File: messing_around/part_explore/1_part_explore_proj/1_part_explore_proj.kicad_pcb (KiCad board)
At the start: 2 copper layers, 8.2 x 5 mm, 2 parts, among them P1 USB_C_Plug_USB2.0, U1 ESP32-C3-WROOM-02

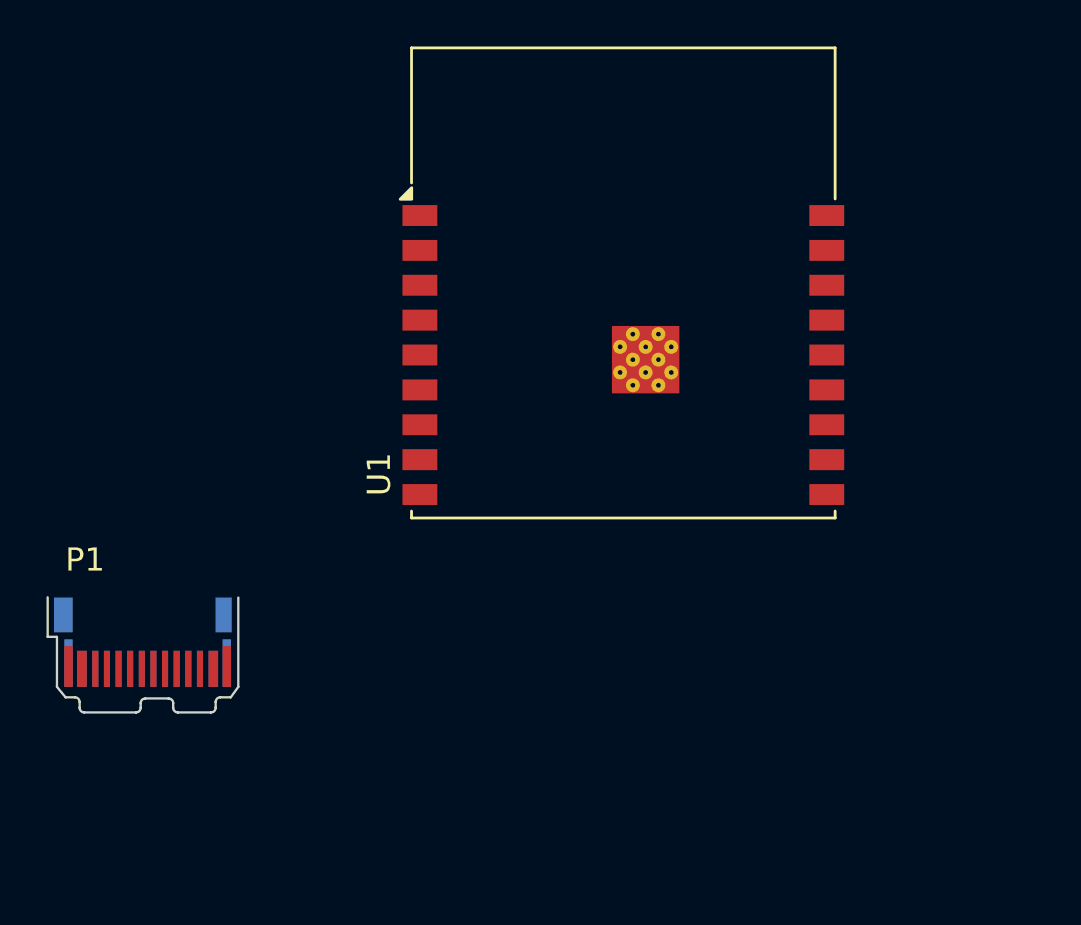
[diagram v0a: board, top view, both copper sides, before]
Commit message: messing around with the settings
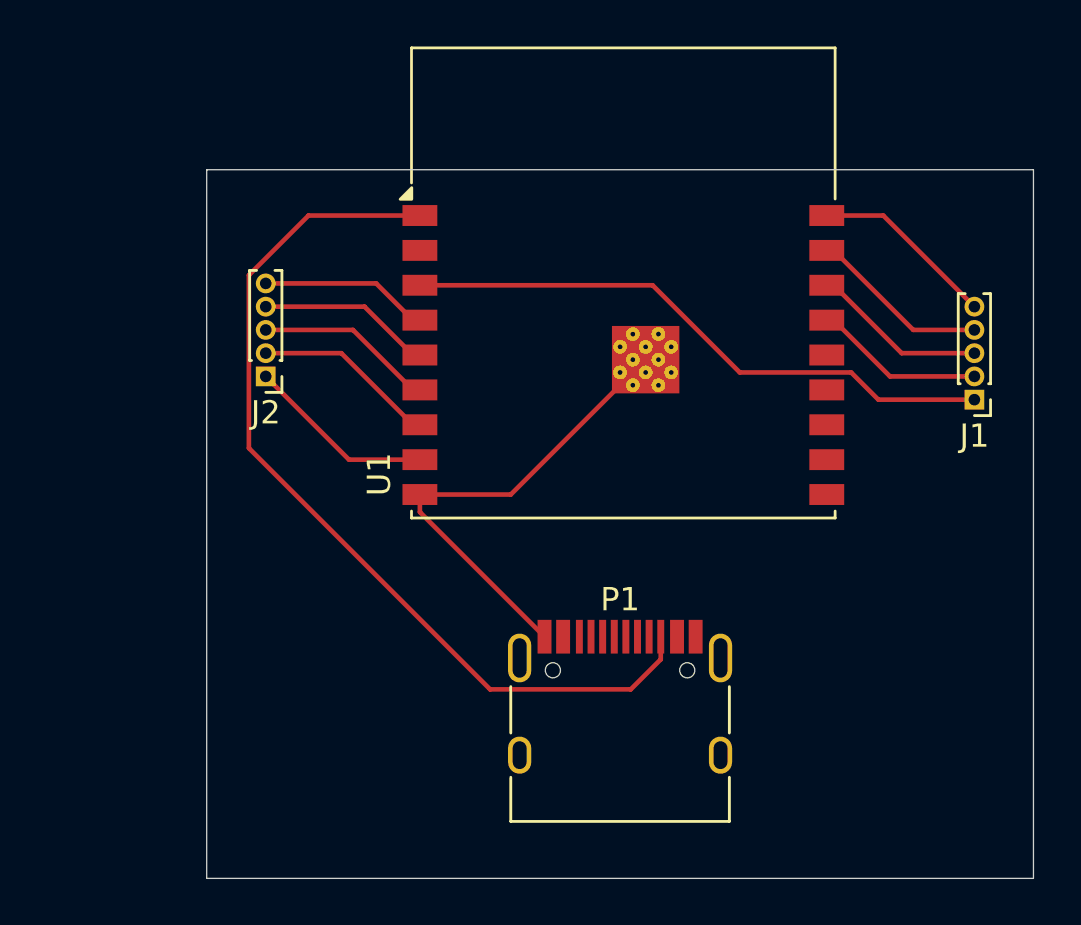
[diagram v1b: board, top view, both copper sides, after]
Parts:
- added J1: Conn_01x05, Connector_PinHeader_1.00mm:PinHeader_1x05_P1.00mm_Vertical, F.Cu at (160.0, 102.6)
- added J2: Conn_01x05, Connector_PinHeader_1.00mm:PinHeader_1x05_P1.00mm_Vertical, F.Cu at (129.5, 101.6)
- P1: footprint Connector_USB:USB_C_Plug_JAE_DX07P024AJ1 -> Connector_USB:USB_C_Receptacle_HRO_TYPE-C-31-M-12
- moved P1 20.7 mm to (144.8, 116.8)
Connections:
- P1 pad A6: Net-(P1-D+) -> /USB_D+
- P1 pad A7: Net-(P1-D-) -> /USB_D-
- U1 pad 13: Net-(P1-D-) -> unconnected-(U1-IO18-Pad13)
- U1 pad 14: Net-(P1-D+) -> unconnected-(U1-IO19-Pad14)
- U1 pad 15: unconnected-(U1-IO3-Pad15) -> /IO_3
- U1 pad 16: unconnected-(U1-IO2-Pad16) -> /IO_2
- U1 pad 17: unconnected-(U1-IO1-Pad17) -> /IO_1
- U1 pad 18: unconnected-(U1-IO0-Pad18) -> /IO_0
- U1 pad 3: unconnected-(U1-IO4-Pad3) -> /IO_4
- U1 pad 4: unconnected-(U1-IO5-Pad4) -> /IO_5
- U1 pad 5: unconnected-(U1-IO6-Pad5) -> /IO_6
- U1 pad 6: unconnected-(U1-IO7-Pad6) -> /IO_7
- U1 pad 7: unconnected-(U1-IO8-Pad7) -> /IO_8
- U1 pad 8: unconnected-(U1-IO9-Pad8) -> /IO_9
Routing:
- net /3.3V: track 0.00 -> 39.4 mm
- net /IO_4: track 0.00 -> 25.9 mm
- net GND: track 0.00 -> 20.4 mm
- net /IO_9: track 0.00 -> 8.11 mm
- net /IO_0: track 0.00 -> 7.97 mm
- net /IO_8: track 0.00 -> 7.91 mm
- net /IO_1: track 0.00 -> 7.77 mm
- net /IO_7: track 0.00 -> 7.70 mm
- net /IO_2: track 0.00 -> 7.56 mm
- net /IO_6: track 0.00 -> 7.49 mm
- net /IO_3: track 0.00 -> 7.35 mm
- net /IO_5: track 0.00 -> 7.28 mm
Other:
- board size 8.2 x 5 mm -> 35.6 x 30.5 mm
